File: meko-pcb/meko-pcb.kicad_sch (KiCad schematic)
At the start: 83 parts, among them IC1 AS5600-ASOM, IC2 TCAL9538RSVR, J1 GDEY0154D67, J2 MEM2090-00-145-00-A, M1 HD-EMB1204-SM, Q1 SS8050, Q2 SS8050, Q3 SS8050, Q4 Si1308EDL, SW1 SW_Push, SW2 SW_Push, SW3 SW_Push, SW4 SW_Push, SW5 SW_Push, SW6 SW_Push, SW7 SW_Push, U1 ESP32-PICO-MINI-02

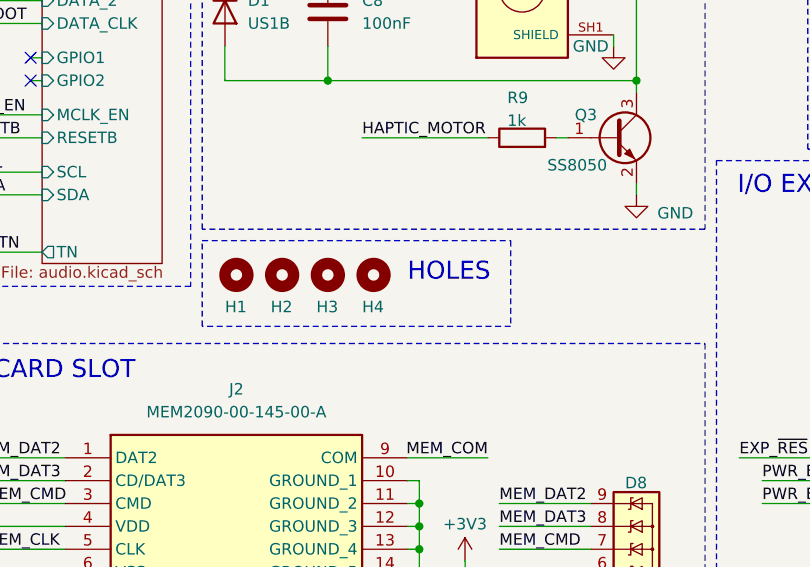
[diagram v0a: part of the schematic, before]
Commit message: 3d stuff, fixes
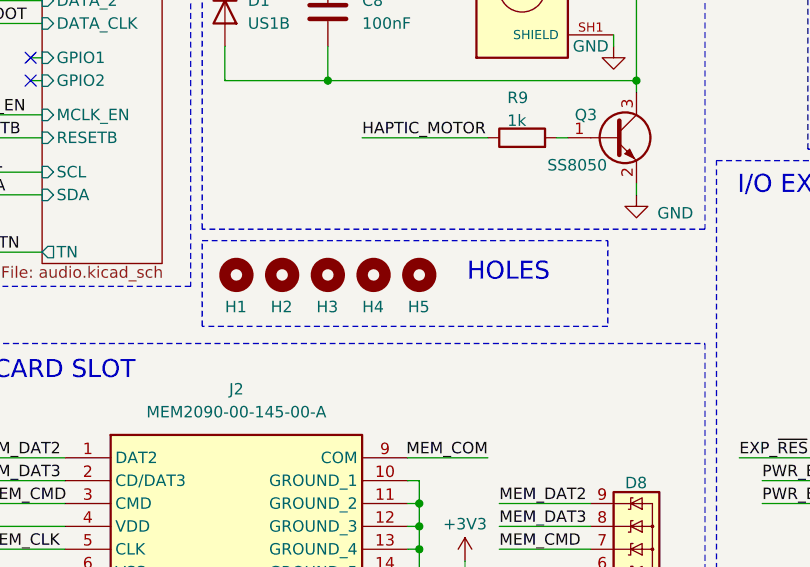
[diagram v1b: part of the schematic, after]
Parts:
- added H5: MountingHole, Library:MountingHole_1.8mm_M1.6, symbol Mechanical:MountingHole
- H1, H2, H3, H4: footprint MountingHole:MountingHole_2.2mm_M2 -> Library:MountingHole_1.8mm_M1.6
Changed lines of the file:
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@@
 	(rectangle
 		(start 50.8 130.81)
-		(end 85.09 140.335)
+		(end 95.885 140.335)
 		(stroke
 			(width 0)
@@
 	(text "HOLES"
 		(exclude_from_sim no)
-		(at 78.232 134.366 0)
+		(at 84.836 134.366 0)
 		(effects
 			(font
@@
 	)
 	(symbol
+		(lib_id "Mechanical:MountingHole")
+		(at 74.93 134.62 0)
+		(unit 1)
+		(exclude_from_sim no)
+		(in_bom no)
+		(on_board yes)
+		(dnp no)
+		(property "Reference" "H5"
+			(at 73.66 138.176 0)
+			(effects
+				(font
+					(size 1.27 1.27)
+				)
+				(justify left)
+			)
+		)
+		(property "Value" "MountingHole"
+			(at 77.47 135.8899 0)
+			(effects
+				(font
+					(size 1.27 1.27)
+				)
+				(justify left)
+				(hide yes)
+			)
+		)
+		(property "Footprint" "Library:MountingHole_1.8mm_M1.6"
+			(at 74.93 134.62 0)
+			(effects
+				(font
+					(size 1.27 1.27)
+				)
+				(hide yes)
+			)
+		)
+		(property "Datasheet" "~"
+			(at 74.93 134.62 0)
+			(effects
+				(font
+					(size 1.27 1.27)
+				)
+				(hide yes)
+			)
+		)
+		(property "Description" "Mounting Hole without connection"
+			(at 74.93 134.62 0)
+			(effects
+				(font
+					(size 1.27 1.27)
+				)
+				(hide yes)
+			)
+		)
+		(instances
+			(project "meko-pcb"
+				(path "/bdd43acd-23c1-472b-909a-8e24eb60d56d"
+					(reference "H5")
+					(unit 1)
+				)
+			)
+		)
+	)
+	(symbol
 		(lib_id "power:+3V3")
 		(at 196.85 111.76 0)
@@
 			)
 		)
-		(property "Footprint" "MountingHole:MountingHole_2.2mm_M2"
+		(property "Footprint" "Library:MountingHole_1.8mm_M1.6"
 			(at 59.69 134.62 0)
 			(effects
@@
 			)
 		)
-		(property "Footprint" "MountingHole:MountingHole_2.2mm_M2"
+		(property "Footprint" "Library:MountingHole_1.8mm_M1.6"
 			(at 69.85 134.62 0)
 			(effects
@@
 			)
 		)
-		(property "Footprint" "MountingHole:MountingHole_2.2mm_M2"
+		(property "Footprint" "Library:MountingHole_1.8mm_M1.6"
 			(at 64.77 134.62 0)
 			(effects
@@
 			)
 		)
-		(property "Footprint" "MountingHole:MountingHole_2.2mm_M2"
+		(property "Footprint" "Library:MountingHole_1.8mm_M1.6"
 			(at 54.61 134.62 0)
 			(effects
